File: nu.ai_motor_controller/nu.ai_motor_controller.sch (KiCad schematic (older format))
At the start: 11 parts

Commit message: cleaned up and renamed project files. Changed custom library management scheme. It now resides in my homedir as a seperate git project, and is pointed to in kicad's symbol library manager
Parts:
- J? (x8): symbol nu-rescue:PTH_1_mm-custom -> custom:PTH_1_mm
- J? (x2): symbol nu-rescue:PTH_3_mm-custom -> custom:PTH_3_mm
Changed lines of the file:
@@
 EESchema Schematic File Version 4
-LIBS:nu-cache
+LIBS:nu.ai_motor_controller-cache
 EELAYER 26 0
 EELAYER END
@@
 $EndComp
 $Comp
-L nu-rescue:PTH_3_mm-custom J?
+L custom:PTH_3_mm J?
 U 1 1 5C162A1D
 P 1250 4200
@@
 $EndComp
 $Comp
-L nu-rescue:PTH_3_mm-custom J?
+L custom:PTH_3_mm J?
 U 1 1 5C162B98
 P 1250 3950
@@
 	-1   0    0    -1
 $EndComp
-Wire Wire Line
-	1400 3950 1850 3950
 Wire Wire Line
 	1400 4200 1750 4200
@@
 	9950 2700 10100 2700
 $Comp
-L nu-rescue:PTH_1_mm-custom J?
+L custom:PTH_1_mm J?
 U 1 1 5C14202A
 P 10550 2200
@@
 $EndComp
 $Comp
-L nu-rescue:PTH_1_mm-custom J?
+L custom:PTH_1_mm J?
 U 1 1 5C1420FB
 P 10550 2400
@@
 $EndComp
 $Comp
-L nu-rescue:PTH_1_mm-custom J?
+L custom:PTH_1_mm J?
 U 1 1 5C142269
 P 10550 2700
@@
 $EndComp
 $Comp
-L nu-rescue:PTH_1_mm-custom J?
+L custom:PTH_1_mm J?
 U 1 1 5C14226F
 P 10550 2900
@@
 $EndComp
 $Comp
-L nu-rescue:PTH_1_mm-custom J?
+L custom:PTH_1_mm J?
 U 1 1 5C1426F8
 P 10550 3200
@@
 $EndComp
 $Comp
-L nu-rescue:PTH_1_mm-custom J?
+L custom:PTH_1_mm J?
 U 1 1 5C1426FE
 P 10550 3400
@@
 $EndComp
 $Comp
-L nu-rescue:PTH_1_mm-custom J?
+L custom:PTH_1_mm J?
 U 1 1 5C142704
 P 10550 3700
@@
 $EndComp
 $Comp
-L nu-rescue:PTH_1_mm-custom J?
+L custom:PTH_1_mm J?
 U 1 1 5C14270A
 P 10550 3900
@@
 F1 "microcontroller.sch" 50
 $EndSheet
+Wire Wire Line
+	1400 3950 1850 3950
 $EndSCHEMATC

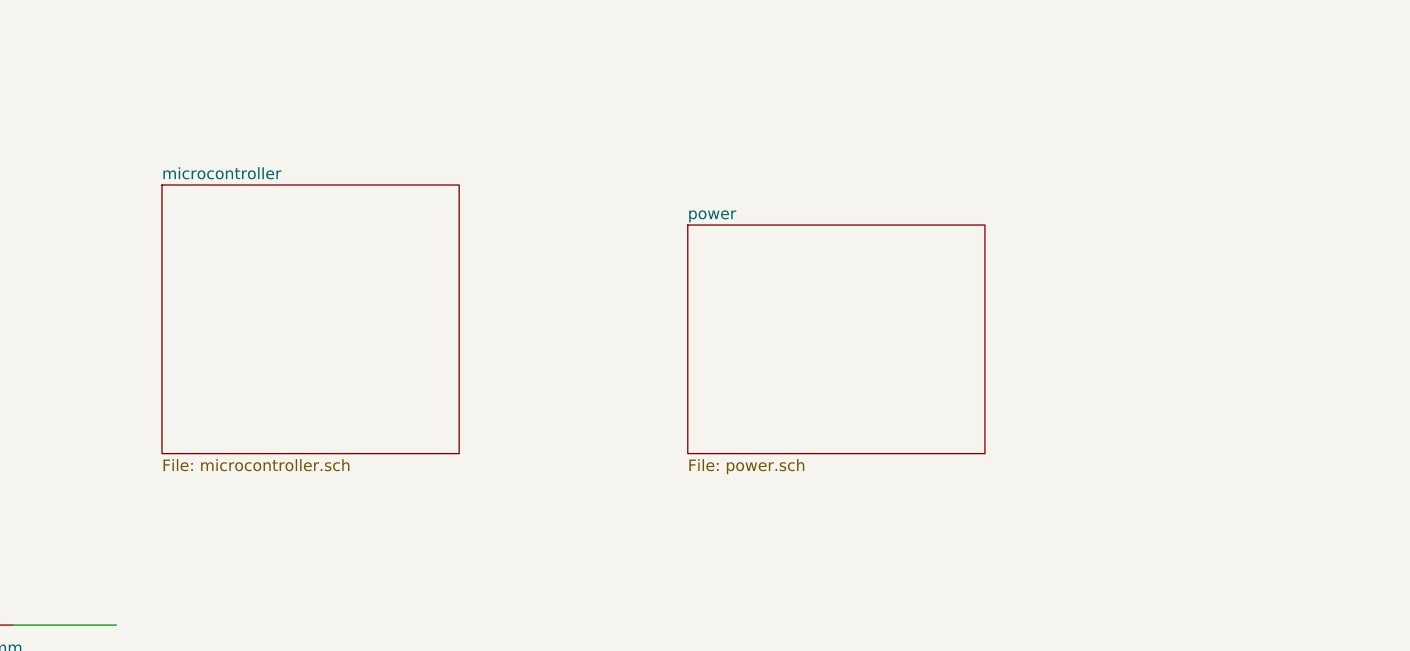
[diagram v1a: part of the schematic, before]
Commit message: automated commit
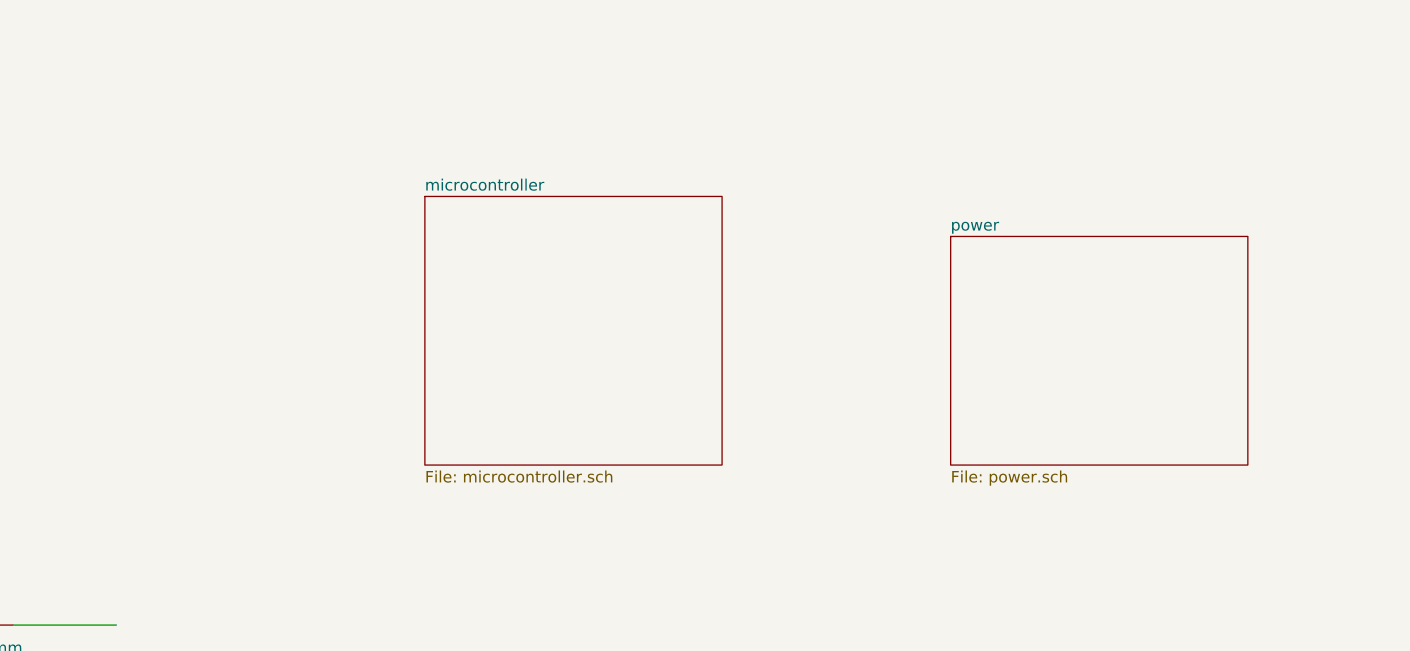
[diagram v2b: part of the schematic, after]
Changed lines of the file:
@@
 $EndDescr
 $Sheet
-S 4350 2200 1300 1000
+S 5500 2250 1300 1000
 U 5C100B31
 F0 "power" 50
@@
 ADD 2 mm STRAIN RELIEF HOLES
 $Sheet
-S 2050 2025 1300 1175
+S 3200 2075 1300 1175
 U 5C3EC885
 F0 "microcontroller" 50
